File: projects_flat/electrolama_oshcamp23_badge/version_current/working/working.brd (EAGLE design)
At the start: 75 x 37 mm, 2 parts

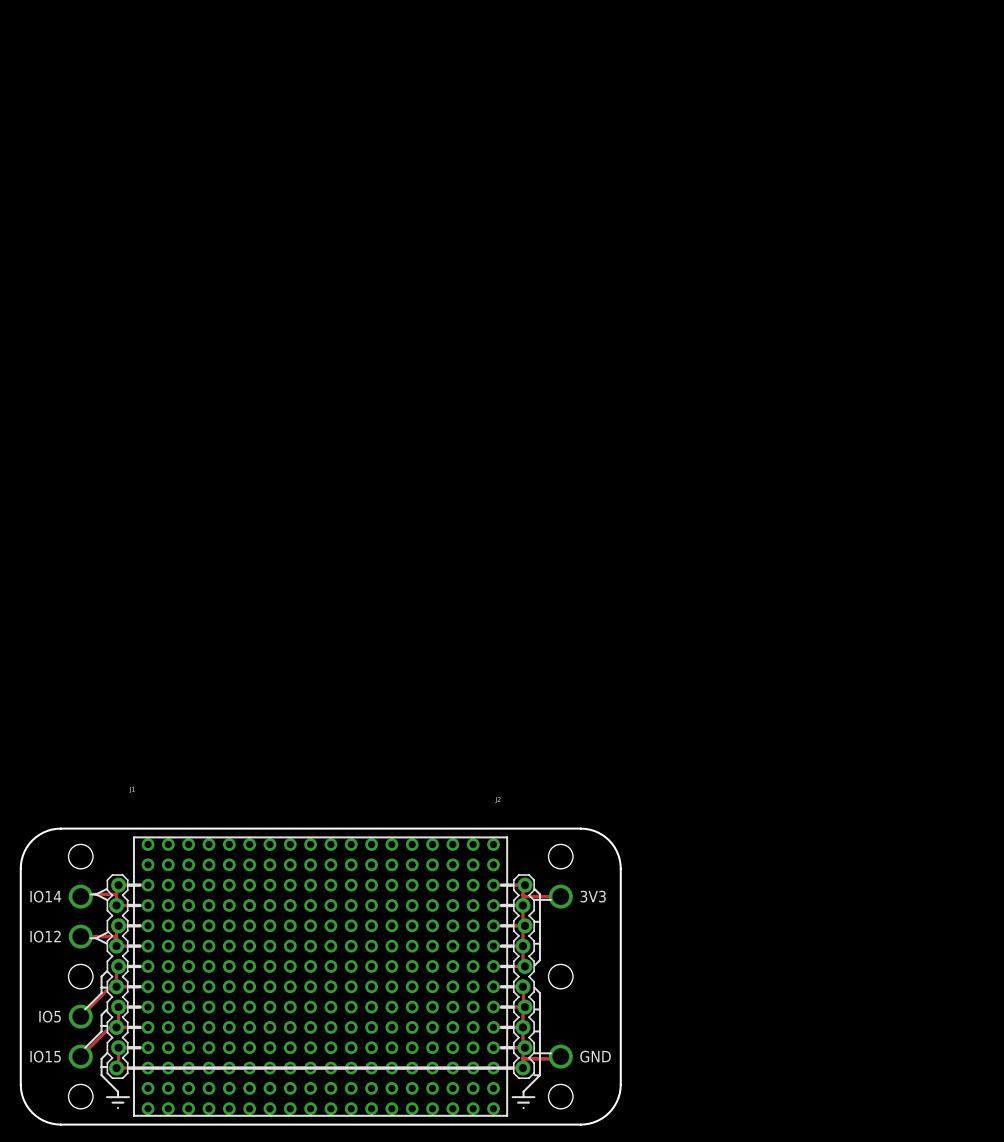
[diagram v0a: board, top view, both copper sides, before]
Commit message: fixed oshcamp pcb
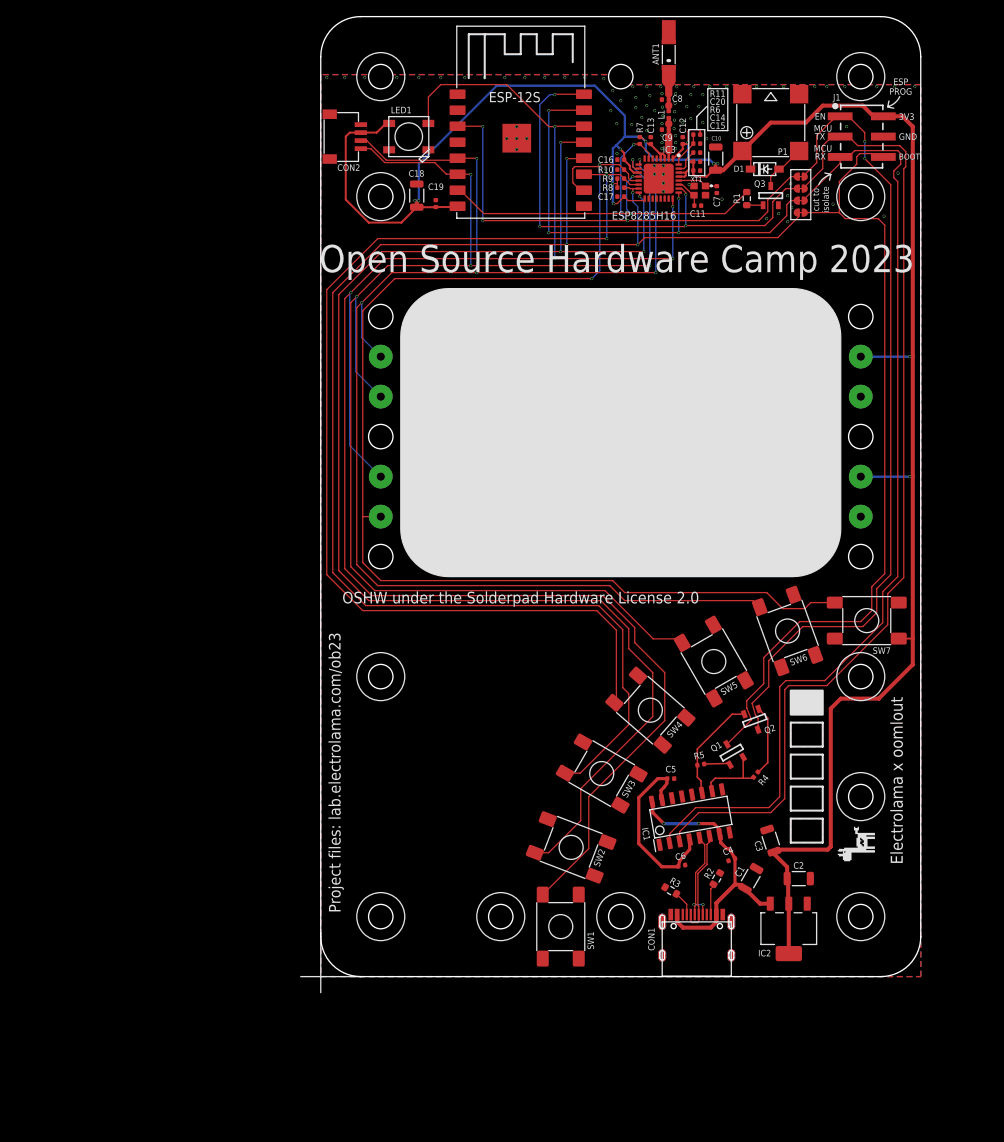
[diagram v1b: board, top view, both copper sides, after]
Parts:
- removed J2: (no value), SparkFun-Connectors:1X10_LOCK
- added ANT1: ANT3216LL00R2400A, ok-rf-dev:YAGEO-ANT3216LL00R2400A
- added C1, C10, C18, C2, C3: 47u, ok-discretes-dev:_PKG_C_1206
- added C11, C7: 8p, ok-discretes-dev:_PKG_C_0402
- added C12, C14: 4u7, ok-discretes-dev:_PKG_C_0402_NOTHERMALS
- added C13, C15, C16, C17, C20: 100n, ok-discretes-dev:_PKG_C_0402_NOTHERMALS
- added C19, C4, C5, C6: 100n, ok-discretes-dev:_PKG_C_0402
- added C8, C9: TBD, ok-discretes-dev:_PKG_C_0402_NOTHERMALS
- added CON1: (no value), ok-connectors-dev:USBC_C-31-M-12
- added CON2: STEMMA_I2C_QT, microbuilder:JST_SH4
- added D1: (no value), ok-discretes-dev:_PKG_SOD123
- added IC1: (no value), ok-chips-dev:_PKG_SOP16
- added IC2: LD1117-3.3, ok-chips-dev:_PKG_SOT223-4_TI-DCY4
- added IC3: WMCU-ESP8285H16, ok-chips-dev:QFN50P500X500X90-33N
- added L1: TBD, ok-discretes-dev:_PKG_L_0402
- added LED1: WS2812B5050, adafruit:WS2812B
- added MOD1: ESP-12S, ok-modules-dev:ESP-12S
- added P1: Buzzer, ok-electromech-dev:MLT-8530
- added Q1, Q2, Q3: SS8050, ok-discretes-dev:SOT96P237X111-3N
- added R1: 220, ok-discretes-dev:_PKG_R_0603
- added R10, R11, R4, R5, R6, R7, R8, R9: 12k 1%, ok-discretes-dev:_PKG_R_0402
- added R2, R3: 5k1, ok-discretes-dev:_PKG_R_0603
- added SJ1, SJ2, SJ3, SJ4: (no value), ok-mechanical-dev:SJ-SHORT
- added SW1, SW2, SW3, SW4, SW5, SW6, SW7: (no value), ok-electromech-dev:GENERIC_SPNO_4P_6X6MM
- added XT1: 26MHz, ok-xtal-osc-dev:XTAL-4P-2016
- J1: value (none) -> 61030621121; device SparkFun-Connectors:1X10_LOCK -> Wurth_Connectors_WR-PHD:61030621121
- moved J1 131.9 mm to (67.6, 105.0)
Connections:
- removed net 3V3: J2.1, J2.2, J2.3, J2.4, J2.5
- new net ANT: C9.2, IC3.2, L1.2
- new net ANT': ANT1.S1, C8.2, L1.1
- new net AUTORST_BOOT: J1.6, Q1.3, SJ4.1
- new net AUTORST_EN: J1.1, Q2.3, SJ1.2
- new net CH343_3V: C5.1, C6.1, IC1.15, IC1.4
- new net DTR: IC1.10, Q1.2, R4.1
- new net EN: IC3.7, MOD1.EN, R7.2, SJ1.1
- new net IO0: IC3.15, MOD1.IO0, R8.2, SJ4.2, SW3.P$1, SW3.P$2
- new net IO13: IC3.12, MOD1.IO13, R1.2
- new net IO1_TX: IC3.26, MOD1.TXD/IO1, SJ2.1
- new net IO2: IC3.14, MOD1.IO2, R9.2, SW4.P$1, SW4.P$2
- new net IO3_RX: IC3.25, MOD1.RXD/IO3, SJ3.1
- new net IO4: IC3.16, MOD1.IO4, SW2.P$1, SW2.P$2
- new net N$12: D1.2, P1.-, Q3.3
- new net N$13: Q2.1, R4.2
- new net N$16: CON1.CC1, R3.2
- new net N$17: CON1.CC2, R2.2
- new net N$23: Q3.1, R1.1
- new net N$5: Q1.1, R5.1
- new net N$6: IC3.31, R6.1
- new net PC_RX: IC1.3, J1.3, SJ2.2
- new net PC_TX: IC1.2, J1.5, SJ3.2
- new net RST_C: C20.2, IC3.32, R11.1
- new net RST_M: MOD1.RST
- new net RTS: IC1.11, Q2.2, R5.2
- new net USB_N: CON1.DN1, CON1.DN2, IC1.6
- new net USB_P: CON1.DP1, CON1.DP2, IC1.5
- new net VCC: C10.1, C12.2, C13.2, C14.2, C15.2, C16.2, C17.2, C18.1, C19.1, C2.1, C3.1, CON2.2, D1.1, IC2.2, IC2.4, IC3.1, IC3.11, IC3.17, IC3.29, IC3.3, IC3.30, IC3.4, J1.2, LED1.1-VDD, MOD1.VCC, P1.+, R11.2, R7.1, R8.1, R9.1, SW7.P$3, SW7.P$4
- new net VUSB: C1.1, C4.1, CON1.VBUS@1, CON1.VBUS@2, IC1.16, IC1.7, IC2.3
- new net XTAL_IN: C7.2, IC3.28, XT1.1
- new net XTAL_OUT: C11.2, IC3.27, XT1.3
- net GND: now also C1.2, C10.2, C11.1, C12.1, C13.1, C14.1, C15.1, C16.1, C17.1, C18.2, C19.2, C2.2, C20.1, C3.2, C4.2, C5.2, C6.2, C7.1, C8.1, C9.1, CON1.GND@1, CON1.GND@2, CON1.P$1, CON1.P$2, CON1.P$3, CON1.P$4, CON1.P$5, CON1.P$6, CON1.P$7, CON1.P$8, CON2.1, IC1.1, IC2.1, IC3.33, J1.4, LED1.3-GND, MOD1.EPAD, MOD1.GND, Q3.2, R10.1, R2.1, R3.1, R6.2, SW1.P$3, SW1.P$4, SW2.P$3, SW2.P$4, SW3.P$3, SW3.P$4, SW4.P$3, SW4.P$4, SW5.P$3, SW5.P$4, SW6.P$3, SW6.P$4, XT1.2, XT1.4; no longer J1.10, J1.9, J2.10, J2.6, J2.7, J2.8, J2.9
- net IO12: now also CON2.4, IC3.10, MOD1.IO12, SW5.P$1, SW5.P$2; no longer J1.3, J1.4
- net IO14: now also CON2.3, IC3.9, MOD1.IO14, SW6.P$1, SW6.P$2; no longer J1.1, J1.2
- net IO15: now also IC3.13, MOD1.IO15, R10.2, SW7.P$1, SW7.P$2; no longer J1.7, J1.8
- net IO5: now also IC3.24, LED1.4-DIN, MOD1.IO5, SW1.P$1, SW1.P$2; no longer J1.5, J1.6
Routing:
- net VCC: track 0.00 -> 294.6 mm, vias 0 -> 13
- net IO5: track 16.5 -> 231.6 mm, vias 3 -> 6
- net IO0: track 0.00 -> 181.6 mm, vias 0 -> 4
- net IO4: track 0.00 -> 174.7 mm, vias 0 -> 4
- net IO14: track 14.9 -> 177.2 mm, vias 3 -> 6
- net IO12: track 14.8 -> 173.8 mm, vias 3 -> 6
- net IO15: track 16.1 -> 153.5 mm
- net IO2: track 0.00 -> 136.9 mm, vias 0 -> 2
- net PC_RX: track 0.00 -> 124.0 mm
- net PC_TX: track 0.00 -> 122.2 mm
- net AUTORST_EN: track 0.00 -> 101.3 mm, vias 0 -> 2
- net AUTORST_BOOT: track 0.00 -> 100.3 mm
- net GND: track 87.7 -> 0.79 mm, vias 24 -> 91
- net EN: track 0.00 -> 71.2 mm, vias 0 -> 4
- net IO1_TX: track 0.00 -> 62.0 mm, vias 0 -> 4
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- added copper zone on layer 1, net GND
- added copper zone on layer 16, net GND
- added copper zone on layer 1, net N$10
- added copper zone on layer 1, net N$3
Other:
- board size 75 x 37 mm -> 75 x 120 mm
- board text added: "BOOT"
- board text added: "CPWG 50 Ohm Params: H=1.2mm, Er=4.6 (FR-4 standard) W=0.92mm, G=0.1524mm Calculated Z=50.0773 Ohms"
- board text added: "EN"
- board text added: "ESP PROG"
- board text added: "ESP8285H16"
- board text added: "Electrolama x oomlout"
- board text added: "MCU"
- board text added: "OSHW under the Solderpad Hardware License 2.0"
- board text added: "Open Source Hardware Camp 2023"
- board text added: "Project files: lab.electrolama.com/ob23"
- board text added: "RX"
- board text added: "TX"
- board text added: "cut to isolate"
- board text removed: "IO12"
- board text removed: "IO14"
- board text removed: "IO15"
- board text removed: "IO5"
- board text removed: "lab.electrolama.com/ob23"
